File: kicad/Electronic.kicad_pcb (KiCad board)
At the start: 2 copper layers, 12 parts, among them J1 BATT, J2 SOLAR, J3 US1881, Q1 IRLZ44N, U1 WeMos_mini, U2 MCP1700x-330xxTO

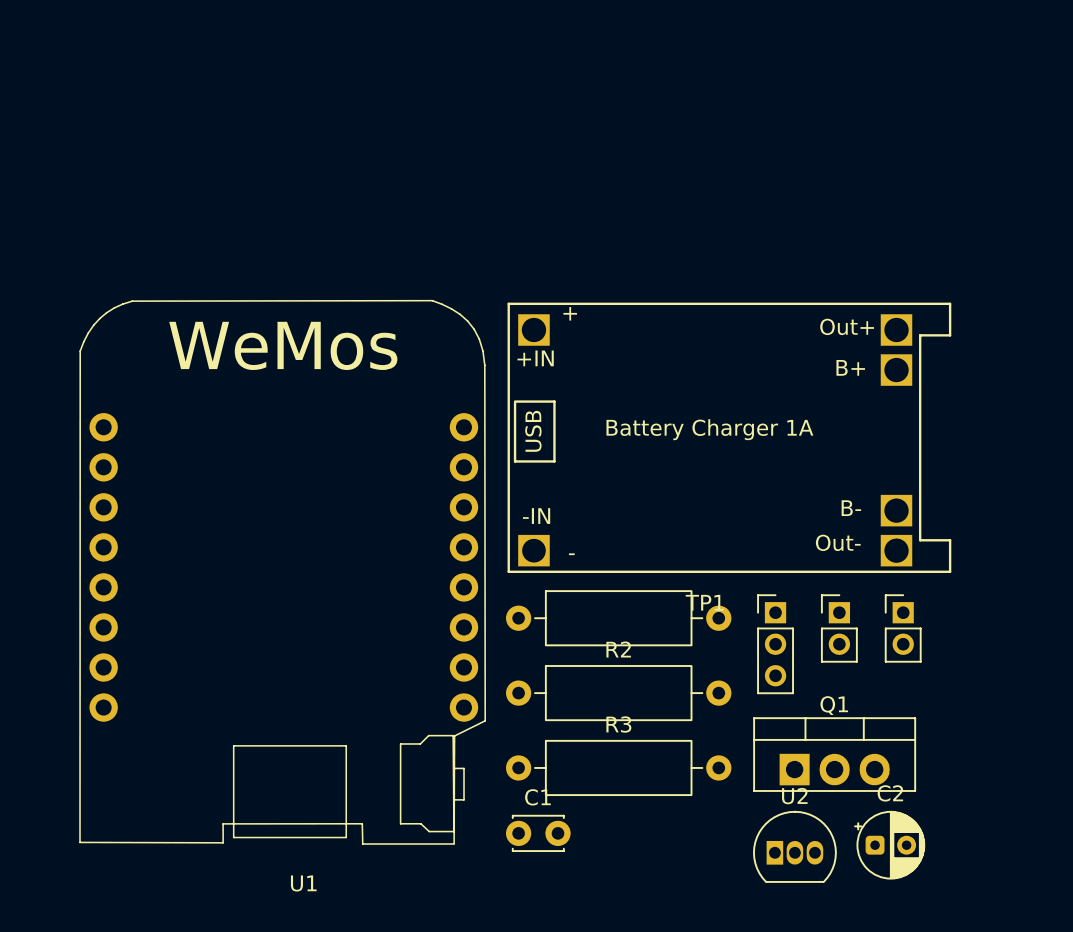
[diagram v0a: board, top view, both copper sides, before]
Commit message: v386 : electronic schematic update
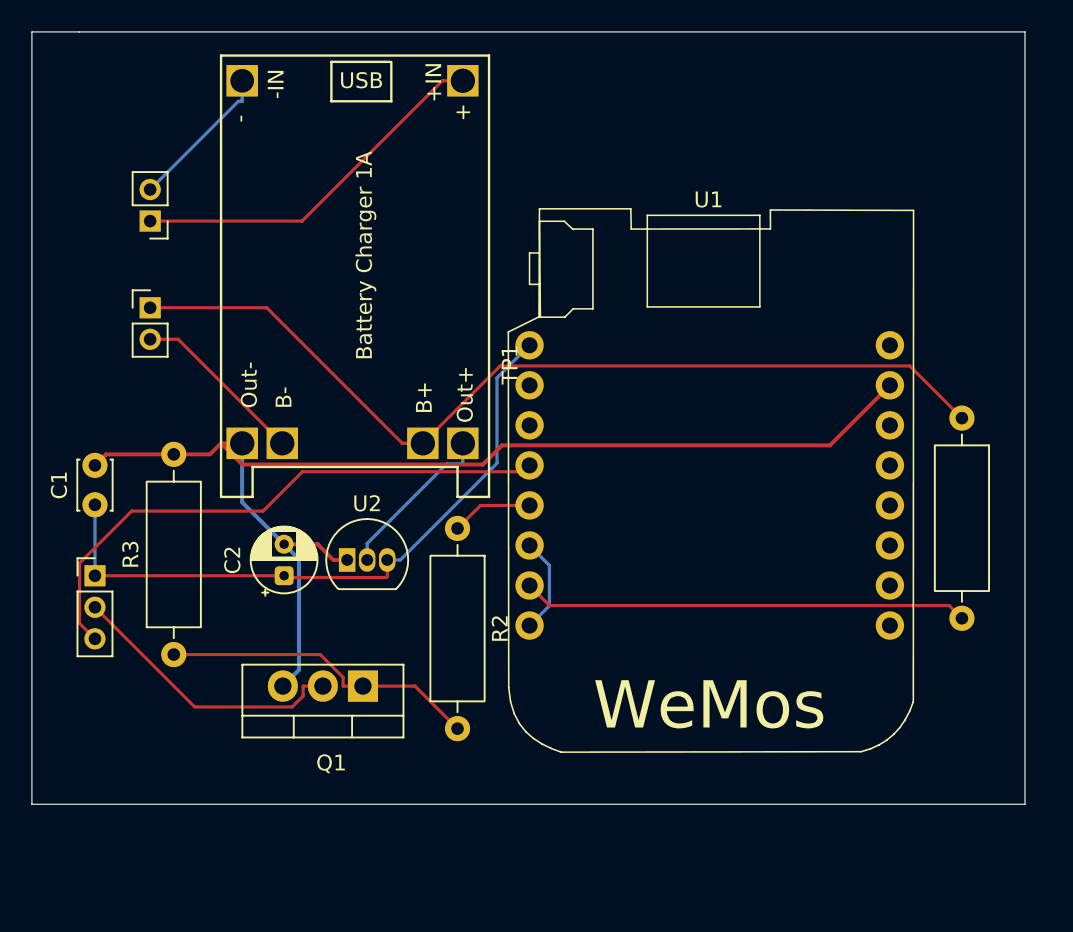
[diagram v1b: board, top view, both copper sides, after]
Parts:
- J1: value BATT -> BAT
- J2: value SOLAR -> SOL
- U2: value MCP1700x-330xxTO -> MCP1700-330
- moved J2 53.8 mm to (118.0, 67.0), turned to 180 degrees
- moved J1 47.8 mm to (118.0, 72.5)
- moved J3 43.2 mm to (114.5, 89.5)
- moved C2 41.2 mm to (126.5, 89.5), turned to 90 degrees
- moved C1 34.0 mm to (114.5, 85.0), turned to 90 degrees
- moved U2 32.9 mm to (130.5, 88.5)
- moved R1 30.9 mm to (169.5, 79.5), turned to -90 degrees
- moved U1 28.1 mm to (153.5, 82.5), turned to 180 degrees
- moved Q1 27.9 mm to (131.5, 96.5), turned to 180 degrees
- moved R3 23.0 mm to (119.5, 94.5), turned to 90 degrees
- moved TP1 15.8 mm to (139.5, 56.5), turned to -90 degrees
- moved R2 11.1 mm to (137.5, 86.5), turned to -90 degrees
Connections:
- TP1 pad 5: /+BAT -> /+VR
- U2 pad 2: /+BAT -> /+VR
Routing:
- net GND: track 0.00 -> 76.7 mm
- net /+BAT: track 0.00 -> 58.5 mm
- net /3.3V: track 0.00 -> 42.0 mm
- net /VIT: track 0.00 -> 36.3 mm
- net Net-(U1-A0): track 0.00 -> 28.3 mm
- net /+SOL: track 0.00 -> 23.5 mm
- net Net-(Q1-G): track 0.00 -> 20.3 mm
- net /-OUT: track 0.00 -> 18.0 mm
- net /-BAT: track 0.00 -> 11.1 mm
- net /+VR: track 0.00 -> 10.5 mm
- net /-SOL: track 0.00 -> 9.46 mm
- net Net-(U1-D0): track 0.00 -> 6.12 mm
- net Net-(U1-D5): track 0.00 -> 5.17 mm
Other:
- board outline added: 63 x 49 mm

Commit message: v386 : electronic schematic update
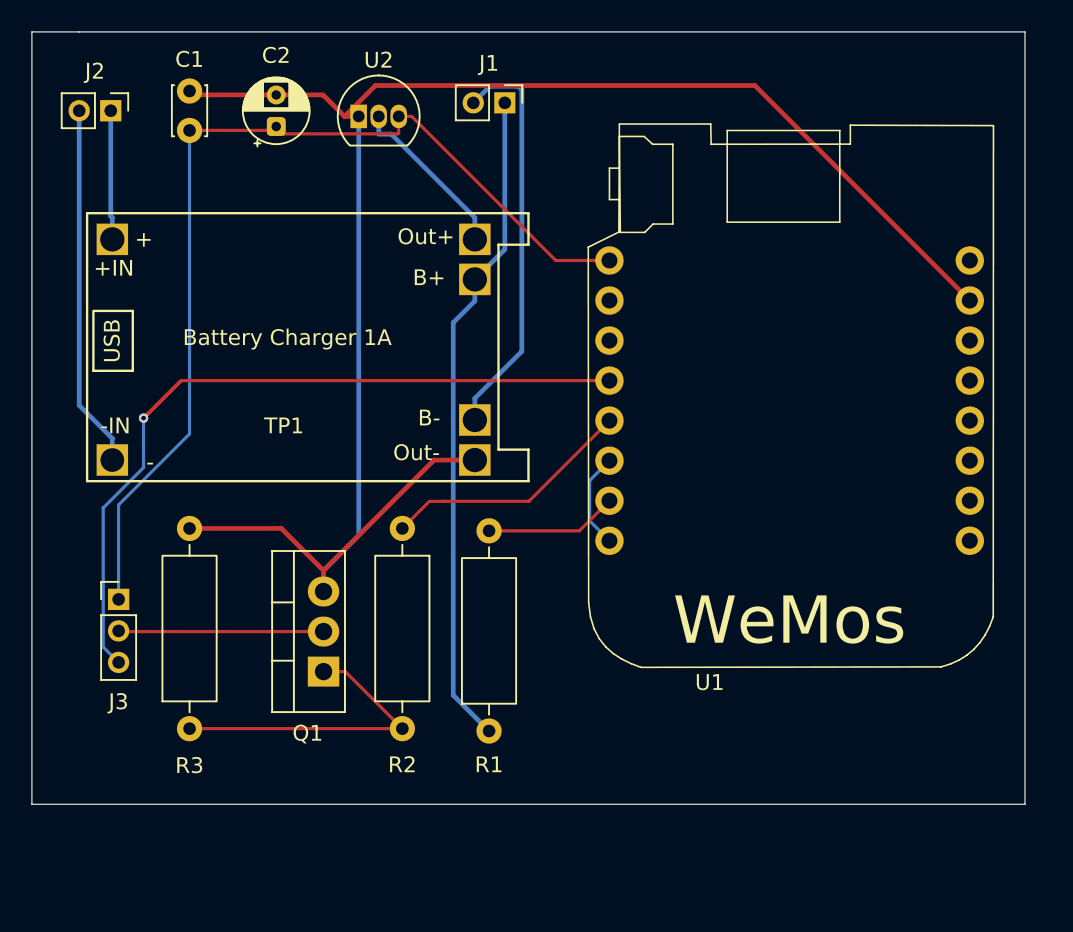
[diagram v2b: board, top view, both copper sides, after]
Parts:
- moved R1 36.0 mm to (139.5, 99.3), turned to 90 degrees
- moved C2 28.5 mm to (126.0, 61.0)
- moved U2 28.1 mm to (131.2, 60.4)
- moved TP1 27.4 mm to (114.0, 66.5), turned to 0 degrees
- moved J1 26.0 mm to (140.5, 59.5), turned to -90 degrees
- moved C1 24.5 mm to (120.5, 61.2)
- moved J2 7.43 mm to (115.5, 60.0), turned to -90 degrees
- moved U1 7.39 mm to (158.6, 77.1)
- moved R3 4.81 mm to (120.5, 99.2)
- moved R2 3.50 mm to (134.0, 86.5)
- moved Q1 2.66 mm to (129.0, 95.6), turned to 90 degrees
- moved J3 2.12 mm to (116.0, 91.0)
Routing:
- net GND: track 76.7 -> 112.0 mm
- net /VIT: track 36.3 -> 60.5 mm, vias 0 -> 1
- net /3.3V: track 42.0 -> 63.4 mm
- net Net-(U1-A0): track 28.3 -> 8.43 mm
- net /+BAT: track 58.5 -> 42.1 mm
- net /+SOL: track 23.5 -> 8.20 mm
- net /-BAT: track 11.1 -> 25.8 mm
- net /-SOL: track 9.46 -> 23.0 mm
- net Net-(U1-D5): track 5.17 -> 16.0 mm
- net /-OUT: track 18.0 -> 13.0 mm

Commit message: v386 : electronic schematic update
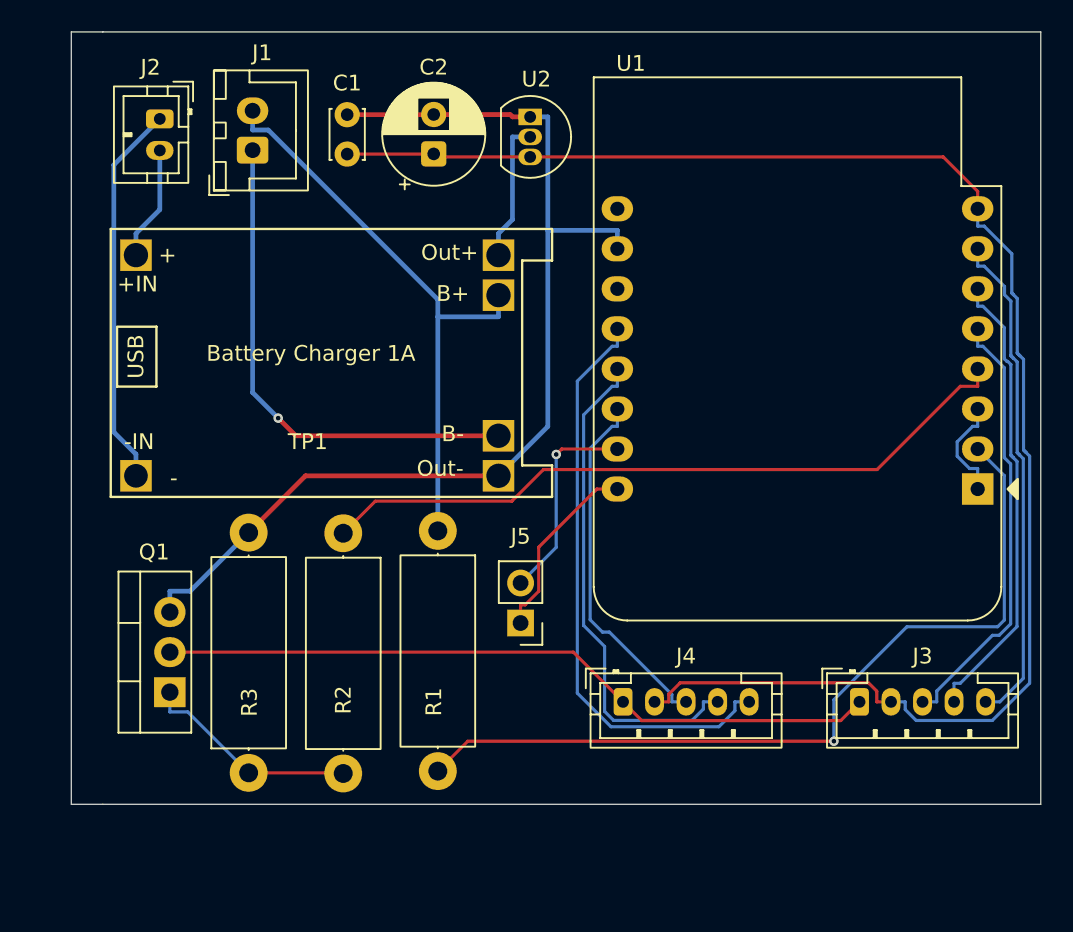
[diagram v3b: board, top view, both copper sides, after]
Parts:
- added J4: GIR, Connector_JST:JST_PH_B5B-PH-K_1x05_P2.00mm_Vertical, F.Cu at (148.0, 97.5)
- added J5: SERIAL, Connector_PinHeader_2.54mm:PinHeader_1x02_P2.54mm_Vertical, F.Cu at (141.5, 92.5)
- C2: footprint Capacitor_THT:CP_Radial_D4.0mm_P2.00mm -> Capacitor_THT:CP_Radial_D6.3mm_P2.50mm
- J1: footprint Connector_PinHeader_2.00mm:PinHeader_1x02_P2.00mm_Vertical -> Connector_JST:JST_XH_B2B-XH-A_1x02_P2.50mm_Vertical
- J2: footprint Connector_PinHeader_2.00mm:PinHeader_1x02_P2.00mm_Vertical -> Connector_JST:JST_PH_B2B-PH-K_1x02_P2.00mm_Vertical
- J3: value US1881 -> ANM; footprint Connector_PinHeader_2.00mm:PinHeader_1x03_P2.00mm_Vertical -> Connector_JST:JST_PH_B5B-PH-K_1x05_P2.00mm_Vertical
- R1, R3: footprint Resistor_THT:R_Axial_DIN0309_L9.0mm_D3.2mm_P12.70mm_Horizontal -> Resistor_THT:R_Axial_DIN0414_L11.9mm_D4.5mm_P15.24mm_Horizontal
- R2: value 220 -> 330; footprint Resistor_THT:R_Axial_DIN0309_L9.0mm_D3.2mm_P12.70mm_Horizontal -> Resistor_THT:R_Axial_DIN0414_L11.9mm_D4.5mm_P15.24mm_Horizontal
- U1: value WeMos_mini -> WeMos_D1_mini_pro; footprint wemos_d1_mini:D1_mini_board -> RF_Module:WEMOS_D1_mini_light
- moved J3 47.4 mm to (163.0, 97.5)
- moved J1 16.3 mm to (124.5, 62.5), turned to 90 degrees
- moved U1 13.8 mm to (170.5, 84.0)
- moved R1 13.1 mm to (136.3, 86.7), turned to -90 degrees
- moved U2 10.9 mm to (142.1, 60.4), turned to -90 degrees
- moved C2 10.1 mm to (136.0, 62.7)
- moved C1 10.1 mm to (130.5, 62.8)
- moved Q1 9.84 mm to (119.3, 96.9)
- moved R3 4.68 mm to (124.3, 102.0)
- moved R2 3.76 mm to (130.3, 86.8)
- moved J2 3.16 mm to (118.6, 60.5)
- moved TP1 1.80 mm to (115.5, 67.5)
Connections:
- J1 pad 1: /+BAT -> /-BAT
- J1 pad 2: /-BAT -> /+BAT
- J2 pad 1: /+SOL -> /-SOL
- J2 pad 2: /-SOL -> /+SOL
- J3 pad 1: /3.3V -> /-OUT
- J3 pad 2: /-OUT -> /3.3V
- U1 pad 1: unconnected-(U1-5V-Pad1) -> Net-(U1-D0)
- U1 pad 10: Net-(U1-A0) -> GND
- U1 pad 11: Net-(U1-D0) -> unconnected-(U1-D4-Pad11)
- U1 pad 12: Net-(U1-D5) -> Net-(J4-Pin_5)
- U1 pad 13: /VIT -> Net-(J4-Pin_4)
- U1 pad 14: unconnected-(U1-D7-Pad14) -> Net-(J4-Pin_3)
- U1 pad 15: unconnected-(U1-D8-Pad15) -> /RX
- U1 pad 16: /3.3V -> /TX
- U1 pad 2: GND -> Net-(U1-A0)
- U1 pad 3: unconnected-(U1-D4-Pad3) -> Net-(U1-D0)
- U1 pad 4: unconnected-(U1-D3-Pad4) -> Net-(U1-D5)
- U1 pad 5: unconnected-(U1-D2-Pad5) -> /VIT
- U1 pad 6: unconnected-(U1-D1-Pad6) -> Net-(J3-Pin_4)
- U1 pad 7: unconnected-(U1-Rx-Pad7) -> Net-(J3-Pin_5)
- U1 pad 8: unconnected-(U1-Tx-Pad8) -> /3.3V
- U1 pad 9: Net-(U1-D0) -> unconnected-(U1-5V-Pad9)
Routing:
- net Net-(U1-A0): track 8.43 -> 53.0 mm, vias 0 -> 1
- net GND: track 112.0 -> 67.7 mm
- net /3.3V: track 63.4 -> 101.6 mm
- net Net-(J4-Pin_5): track 0.00 -> 37.1 mm
- net /-OUT: track 13.0 -> 46.0 mm
- net /VIT: track 60.5 -> 27.8 mm, vias 1 -> 0
- net Net-(J3-Pin_5): track 0.00 -> 32.2 mm
- net Net-(J4-Pin_4): track 0.00 -> 31.5 mm
- net Net-(J3-Pin_4): track 0.00 -> 29.6 mm
- net Net-(U1-D5): track 16.0 -> 45.2 mm
- net Net-(J4-Pin_3): track 0.00 -> 22.8 mm
- net /RX: track 0.00 -> 13.1 mm, vias 0 -> 1
- net /TX: track 0.00 -> 12.0 mm
- net /-BAT: track 25.8 -> 32.1 mm, vias 0 -> 1
- net Net-(Q1-G): track 20.0 -> 13.9 mm
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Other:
- board size 63 x 49 mm -> 61.5 x 49 mm
